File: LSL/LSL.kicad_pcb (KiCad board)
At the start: 2 copper layers, 61 x 26.7 mm, 11 parts, among them J1 Conn_01x01_Male, J2 Conn_01x08_Male, J3 Conn_01x08_Male, J4 Conn_01x01_Male, J5 Conn_01x05_Male, U1 74HC00, U2 74LS573

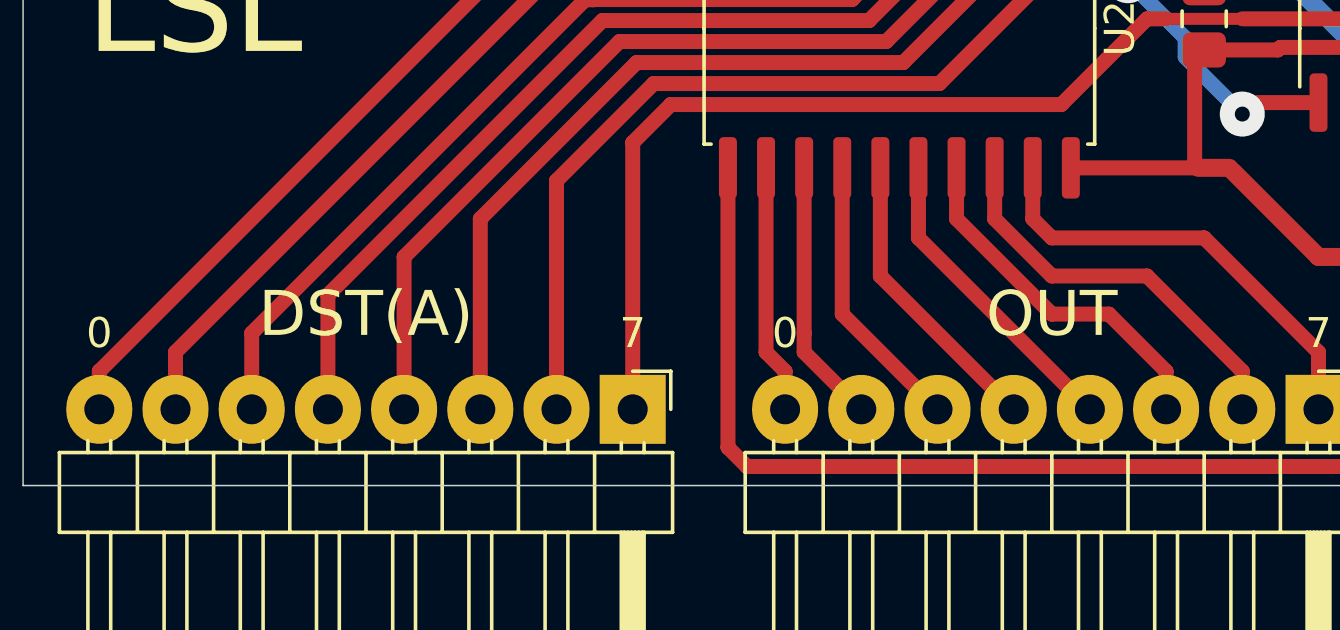
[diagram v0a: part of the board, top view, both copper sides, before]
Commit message: Fix fonts
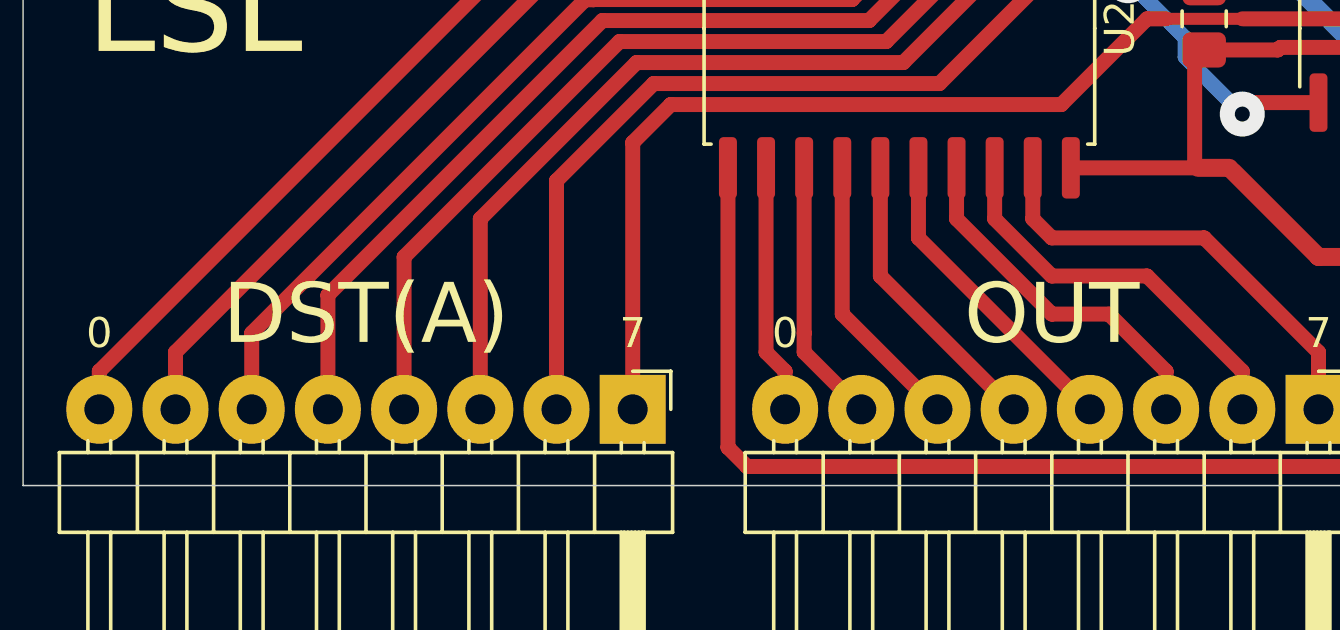
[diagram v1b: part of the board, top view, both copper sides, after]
